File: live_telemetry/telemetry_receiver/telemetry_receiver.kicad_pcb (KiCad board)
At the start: 2 copper layers, 44.8 x 28 mm, 20 parts, among them J1 Conn_Coaxial, J2 Programming Header, J3 USB_A, U1 PIC16LF1455, U2 RFM95W, U3 AP2114H-3.3

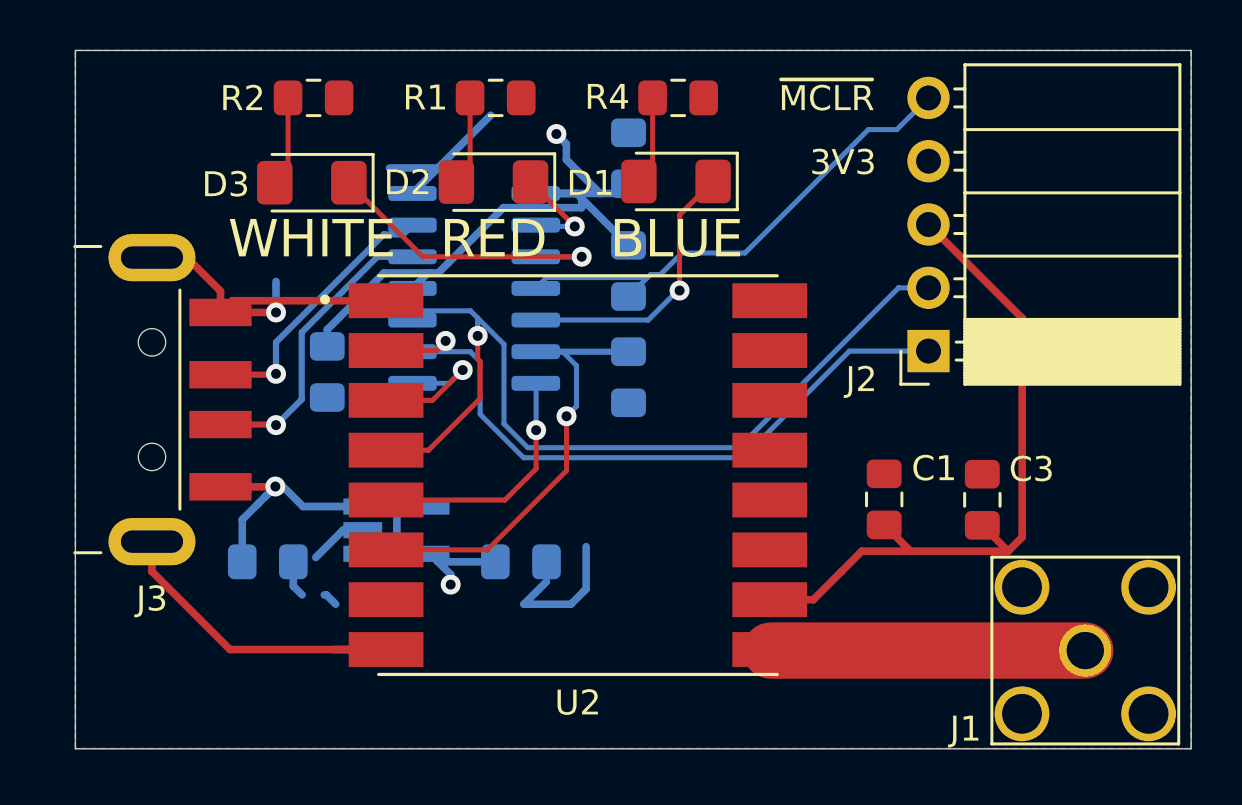
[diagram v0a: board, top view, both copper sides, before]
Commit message: Address Aaron's comments
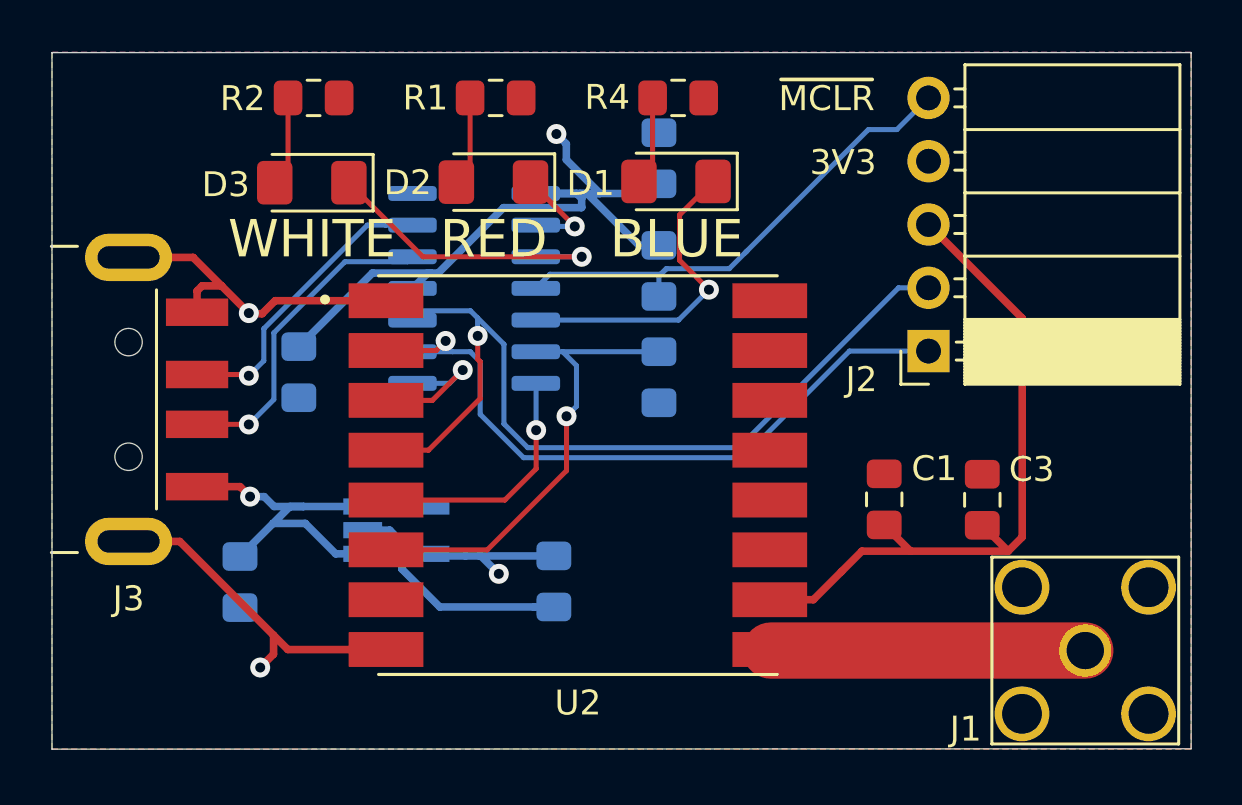
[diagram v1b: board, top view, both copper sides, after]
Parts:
- moved C6 1.54 mm to (127.2, 95.8), turned to 270 degrees
- moved C5 1.38 mm to (114.6, 95.8), turned to 270 degrees
- moved C2 1.22 mm to (131.4, 78.8)
- moved R3 1.22 mm to (131.4, 83.3)
- moved R5 1.22 mm to (131.4, 87.6)
- moved C4 1.14 mm to (116.9, 87.4)
- moved J3 0.94 mm to (103.2, 88.5)
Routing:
- net GND: track 77.6 -> 67.3 mm, vias 1 -> 2
- net +3V3: track 30.2 -> 35.6 mm
- net Net-(D1-Pad1): track 11.2 -> 12.8 mm
- net /USB_D+: track 10.9 -> 11.9 mm
- net /USB_D-: track 12.1 -> 13.0 mm
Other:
- board size 44.8 x 28 mm -> 45.7 x 28 mm

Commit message: Address Alex's comments
Note:
-Still need to pick names for the boards
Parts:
- added G***: LOGO, Team logo:Logo_SilkScreen_5mm, B.Cu at (138.7, 92.5)
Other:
- board text added: "*INSERT NAME* D. Kletke 2020-02-23"
